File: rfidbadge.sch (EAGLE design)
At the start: 51 parts, among them Q1 BSS123, U1 ATMEGA328P_TQFP, U2 CLRC663, Y1 27.12 MHz

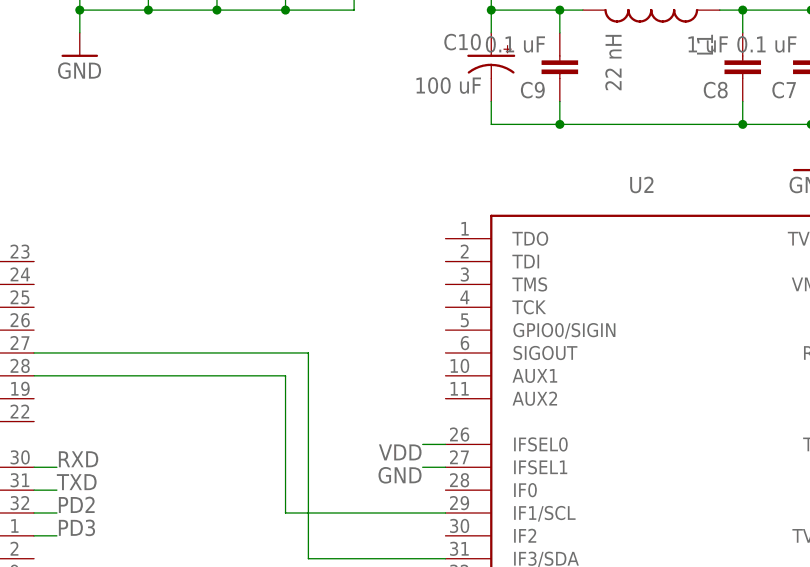
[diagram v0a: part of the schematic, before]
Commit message: Added some test pads
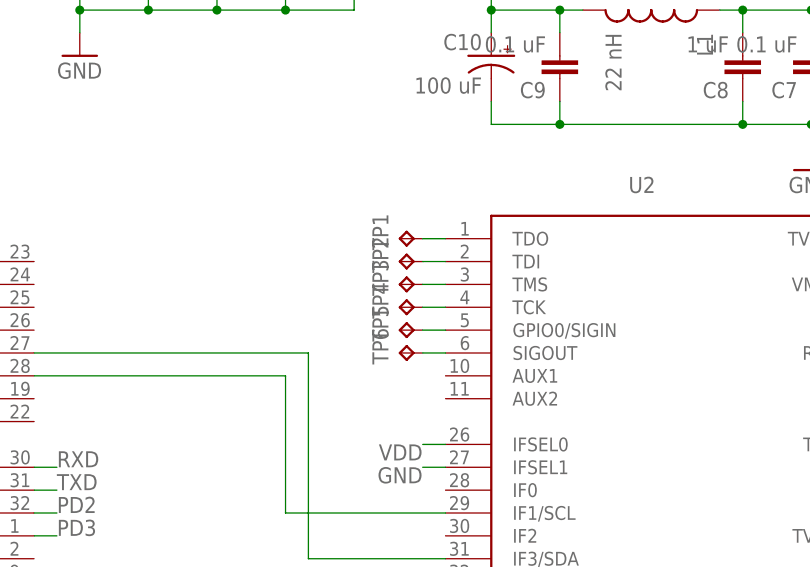
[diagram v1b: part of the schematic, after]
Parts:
- added TP1, TP2, TP3, TP4, TP5, TP6: TPTP06R, testpad:TPTP06R
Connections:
- new net N$12: TP3.TP, U2.TMS
- new net N$13: TP4.TP, U2.TCK
- new net N$14: TP5.TP, U2.GPIO0/SIGIN
- new net N$15: TP6.TP, U2.SIGOUT
- new net N$5: TP1.TP, U2.TDO
- new net N$6: TP2.TP, U2.TDI
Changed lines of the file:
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@@
 <part name="S2" library="SparkFun-Electromechanical" deviceset="SWITCH-MOMENTARY-2" device="SMD-4"/>
 <part name="GND11" library="supply1" deviceset="GND" device=""/>
+<part name="TP1" library="testpad" deviceset="TP" device="TP06R" value="TPTP06R"/>
+<part name="TP2" library="testpad" deviceset="TP" device="TP06R" value="TPTP06R"/>
+<part name="TP3" library="testpad" deviceset="TP" device="TP06R" value="TPTP06R"/>
+<part name="TP4" library="testpad" deviceset="TP" device="TP06R" value="TPTP06R"/>
+<part name="TP5" library="testpad" deviceset="TP" device="TP06R" value="TPTP06R"/>
+<part name="TP6" library="testpad" deviceset="TP" device="TP06R" value="TPTP06R"/>
 </parts>
 <sheets>
@@
 <instance part="S2" gate="G$1" x="157.48" y="71.12"/>
 <instance part="GND11" gate="1" x="165.1" y="66.04"/>
+<instance part="TP1" gate="G$1" x="63.5" y="33.02" rot="R90"/>
+<instance part="TP2" gate="G$1" x="63.5" y="30.48" rot="R90"/>
+<instance part="TP3" gate="G$1" x="63.5" y="27.94" rot="R90"/>
+<instance part="TP4" gate="G$1" x="63.5" y="25.4" rot="R90"/>
+<instance part="TP5" gate="G$1" x="63.5" y="22.86" rot="R90"/>
+<instance part="TP6" gate="G$1" x="63.5" y="20.32" rot="R90"/>
 </instances>
 <busses>
@@
 </segment>
 </net>
+<net name="N$5" class="0">
+<segment>
+<pinref part="U2" gate="G$1" pin="TDO"/>
+<wire x1="66.04" y1="33.02" x2="68.58" y2="33.02" width="0.1524" layer="91"/>
+<pinref part="TP1" gate="G$1" pin="TP"/>
+</segment>
+</net>
+<net name="N$6" class="0">
+<segment>
+<pinref part="U2" gate="G$1" pin="TDI"/>
+<wire x1="68.58" y1="30.48" x2="66.04" y2="30.48" width="0.1524" layer="91"/>
+<pinref part="TP2" gate="G$1" pin="TP"/>
+</segment>
+</net>
+<net name="N$12" class="0">
+<segment>
+<pinref part="U2" gate="G$1" pin="TMS"/>
+<wire x1="68.58" y1="27.94" x2="66.04" y2="27.94" width="0.1524" layer="91"/>
+<pinref part="TP3" gate="G$1" pin="TP"/>
+</segment>
+</net>
+<net name="N$13" class="0">
+<segment>
+<pinref part="U2" gate="G$1" pin="TCK"/>
+<wire x1="68.58" y1="25.4" x2="66.04" y2="25.4" width="0.1524" layer="91"/>
+<pinref part="TP4" gate="G$1" pin="TP"/>
+</segment>
+</net>
+<net name="N$14" class="0">
+<segment>
+<pinref part="U2" gate="G$1" pin="GPIO0/SIGIN"/>
+<wire x1="68.58" y1="22.86" x2="66.04" y2="22.86" width="0.1524" layer="91"/>
+<pinref part="TP5" gate="G$1" pin="TP"/>
+</segment>
+</net>
+<net name="N$15" class="0">
+<segment>
+<pinref part="U2" gate="G$1" pin="SIGOUT"/>
+<wire x1="68.58" y1="20.32" x2="66.04" y2="20.32" width="0.1524" layer="91"/>
+<pinref part="TP6" gate="G$1" pin="TP"/>
+</segment>
+</net>
